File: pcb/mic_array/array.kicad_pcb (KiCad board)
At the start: 4 copper layers, 179.6 x 161 mm, 266 parts, among them J1 M55-7002042R, J2 M55-7002042R, M0 SPH0641LU4H-1, M1 SPH0641LU4H-1, M10 SPH0641LU4H-1, M11 SPH0641LU4H-1, M12 SPH0641LU4H-1, M13 SPH0641LU4H-1, M14 SPH0641LU4H-1, M15 SPH0641LU4H-1, M16 SPH0641LU4H-1, M17 SPH0641LU4H-1, M18 SPH0641LU4H-1, M19 SPH0641LU4H-1, M2 SPH0641LU4H-1, M20 SPH0641LU4H-1, M21 SPH0641LU4H-1, M22 SPH0641LU4H-1, M23 SPH0641LU4H-1, M24 SPH0641LU4H-1, M25 SPH0641LU4H-1, M26 SPH0641LU4H-1, M27 SPH0641LU4H-1, M28 SPH0641LU4H-1, M29 SPH0641LU4H-1, M3 SPH0641LU4H-1, M30 SPH0641LU4H-1, M31 SPH0641LU4H-1, M32 SPH0641LU4H-1, M33 SPH0641LU4H-1, M34 SPH0641LU4H-1, M35 SPH0641LU4H-1, M36 SPH0641LU4H-1, M37 SPH0641LU4H-1, M38 SPH0641LU4H-1, M39 SPH0641LU4H-1, M4 SPH0641LU4H-1, M40 SPH0641LU4H-1, M41 SPH0641LU4H-1, M42 SPH0641LU4H-1, M43 SPH0641LU4H-1, M44 SPH0641LU4H-1, M45 SPH0641LU4H-1, M46 SPH0641LU4H-1, M47 SPH0641LU4H-1, M48 SPH0641LU4H-1, M49 SPH0641LU4H-1, M5 SPH0641LU4H-1, M50 SPH0641LU4H-1, M51 SPH0641LU4H-1, M52 SPH0641LU4H-1, M53 SPH0641LU4H-1, M54 SPH0641LU4H-1, M55 SPH0641LU4H-1, M56 SPH0641LU4H-1, M57 SPH0641LU4H-1, M58 SPH0641LU4H-1, M59 SPH0641LU4H-1, M6 SPH0641LU4H-1, M7 SPH0641LU4H-1, M8 SPH0641LU4H-1, M9 SPH0641LU4H-1

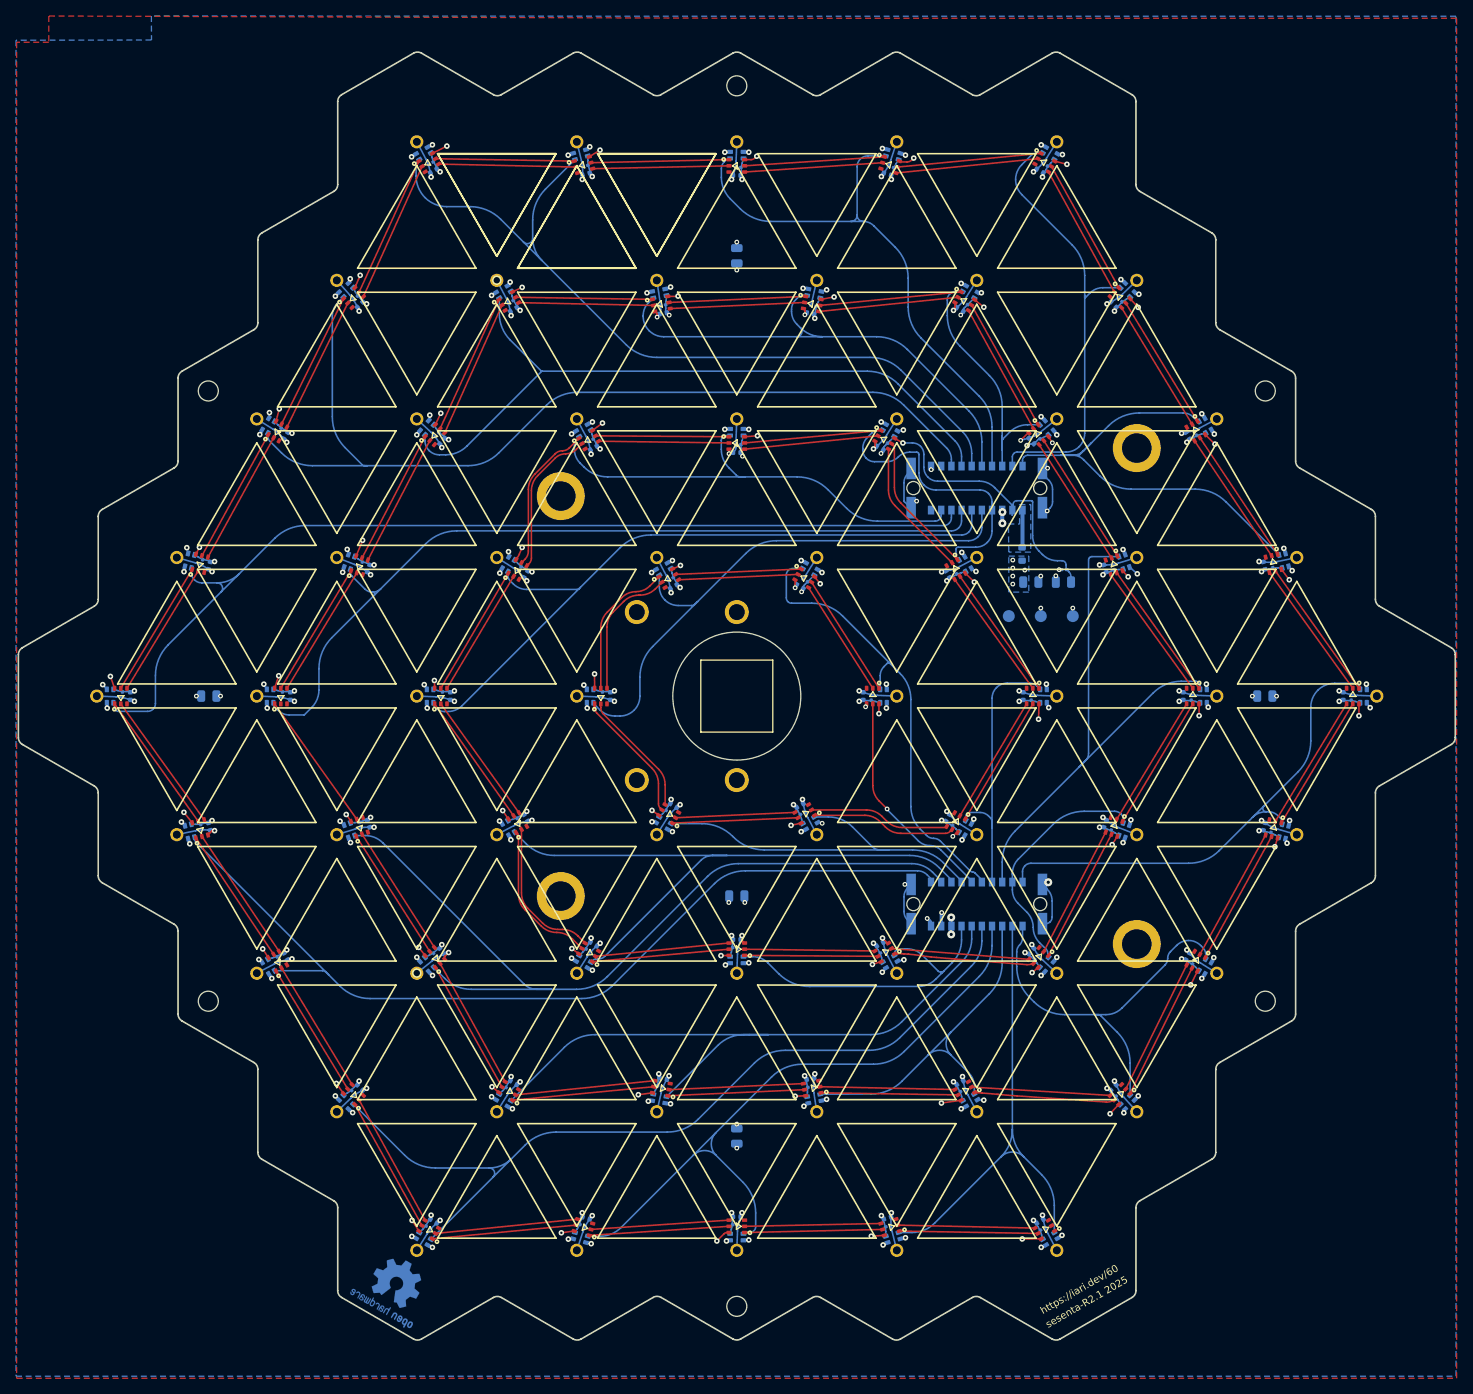
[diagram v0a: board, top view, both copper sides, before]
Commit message: JLCPCB ready
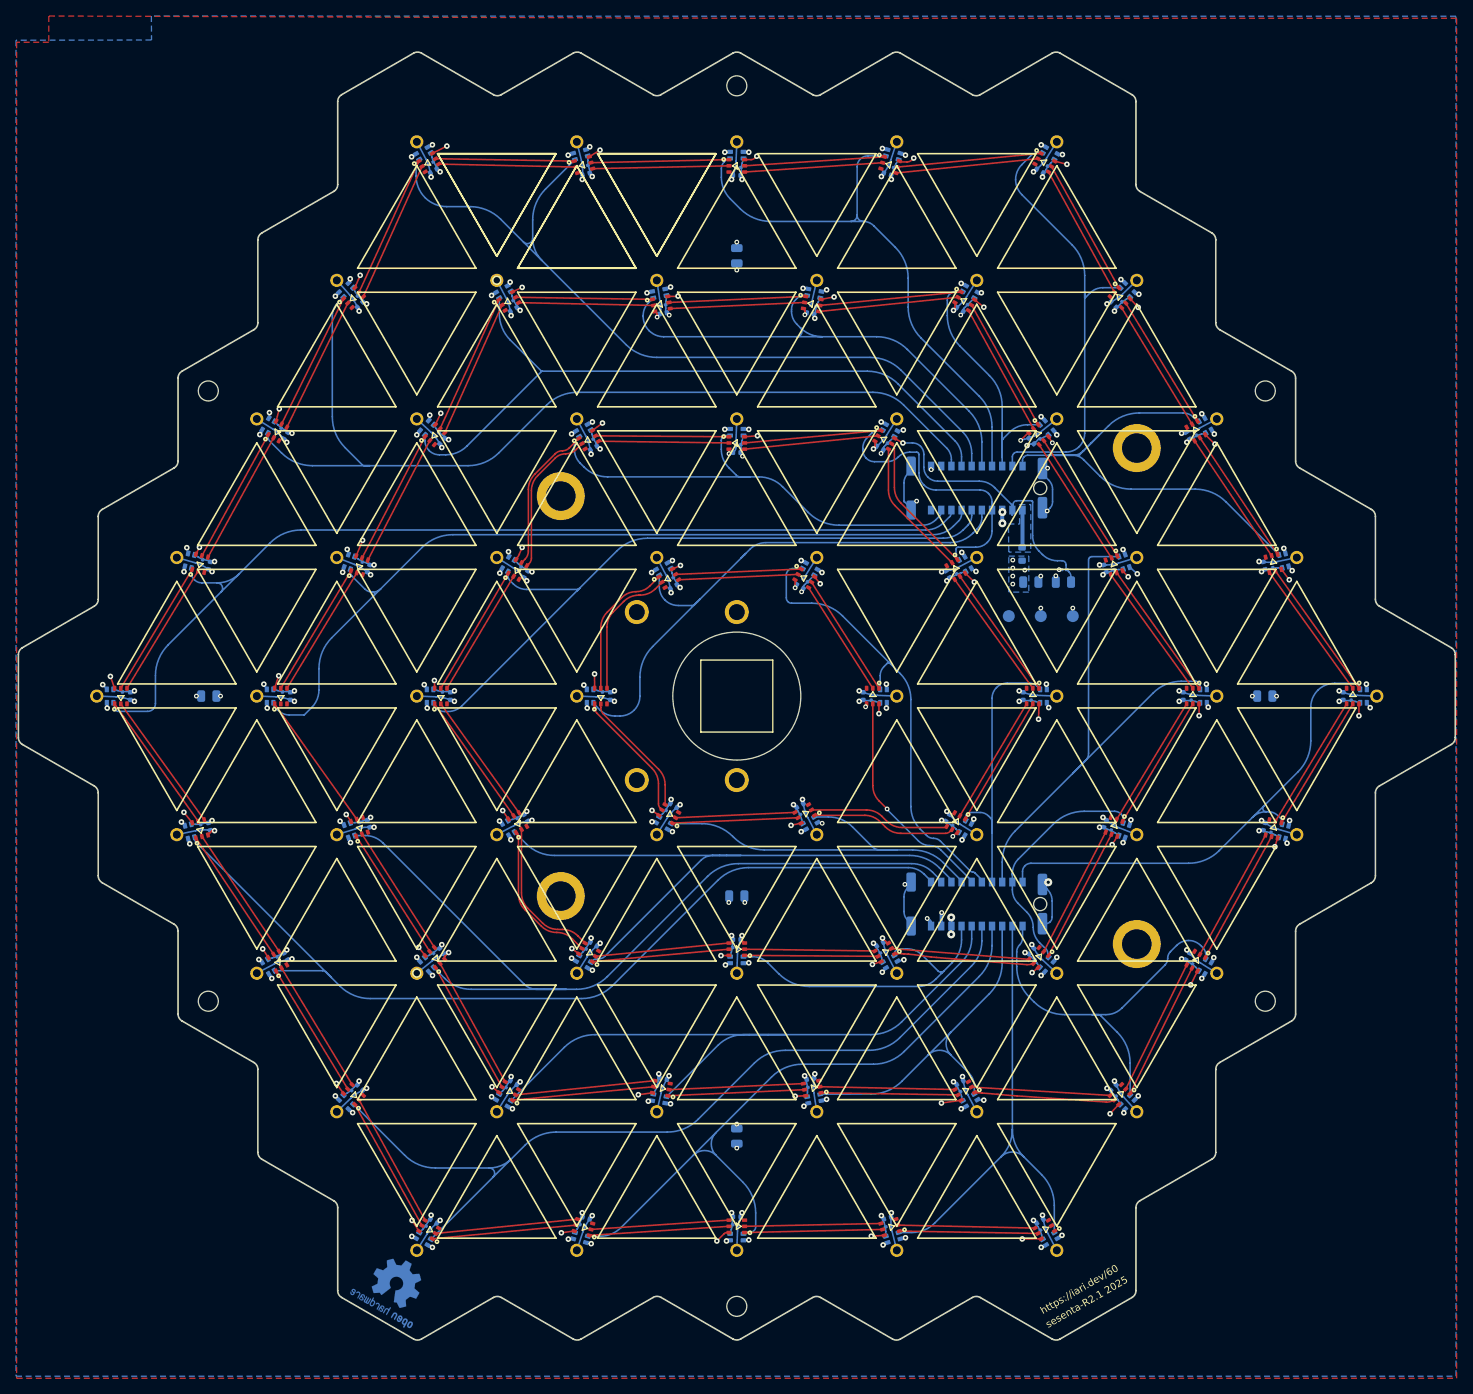
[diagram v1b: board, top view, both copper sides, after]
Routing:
- net /D40: track 59.1 -> 62.1 mm
- net /D32: track 83.5 -> 85.9 mm
- net /D30: track 103.3 -> 105.2 mm
- net /D14: track 78.9 -> 80.7 mm
- net /D22: track 33.1 -> 34.3 mm
- net /D20: track 68.6 -> 69.7 mm
- net /D4: track 49.2 -> 50.3 mm
- net /D52: track 113.8 -> 114.8 mm
- net /D10: track 59.6 -> 60.4 mm
- net /D6: track 35.6 -> 36.3 mm
- net /D2: track 71.5 -> 72.2 mm
- net /D28: track 107.2 -> 106.6 mm
